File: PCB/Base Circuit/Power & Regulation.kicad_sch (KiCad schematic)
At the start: 25 parts, among them SW1_ESTOP SW_SPST

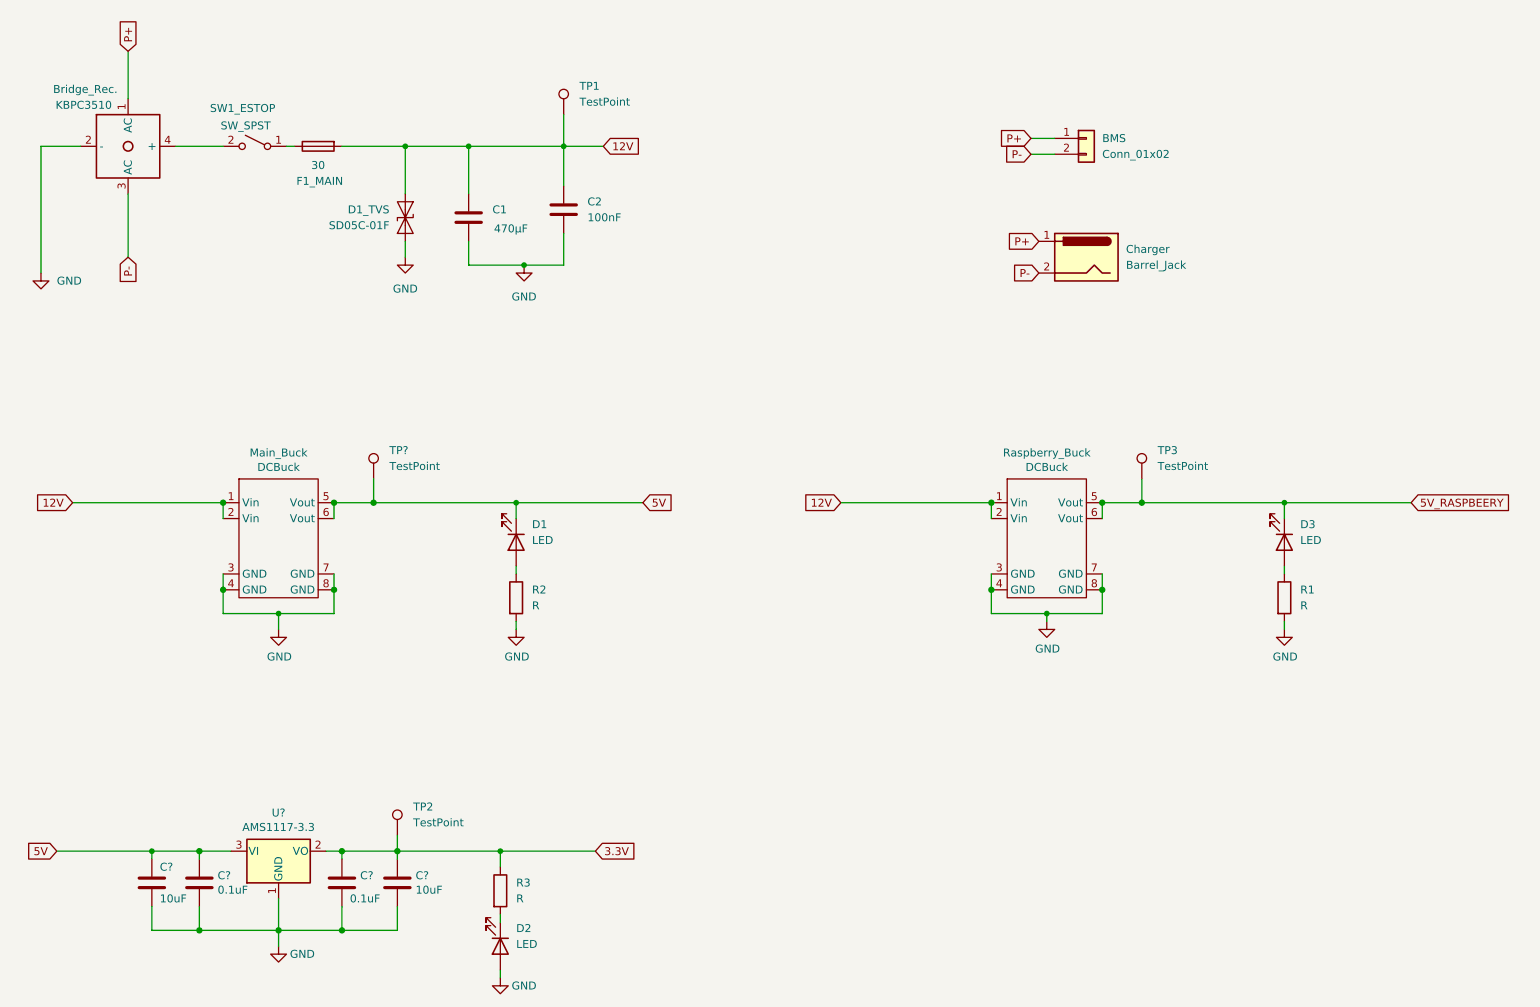
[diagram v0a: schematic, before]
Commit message: Final schematic updated
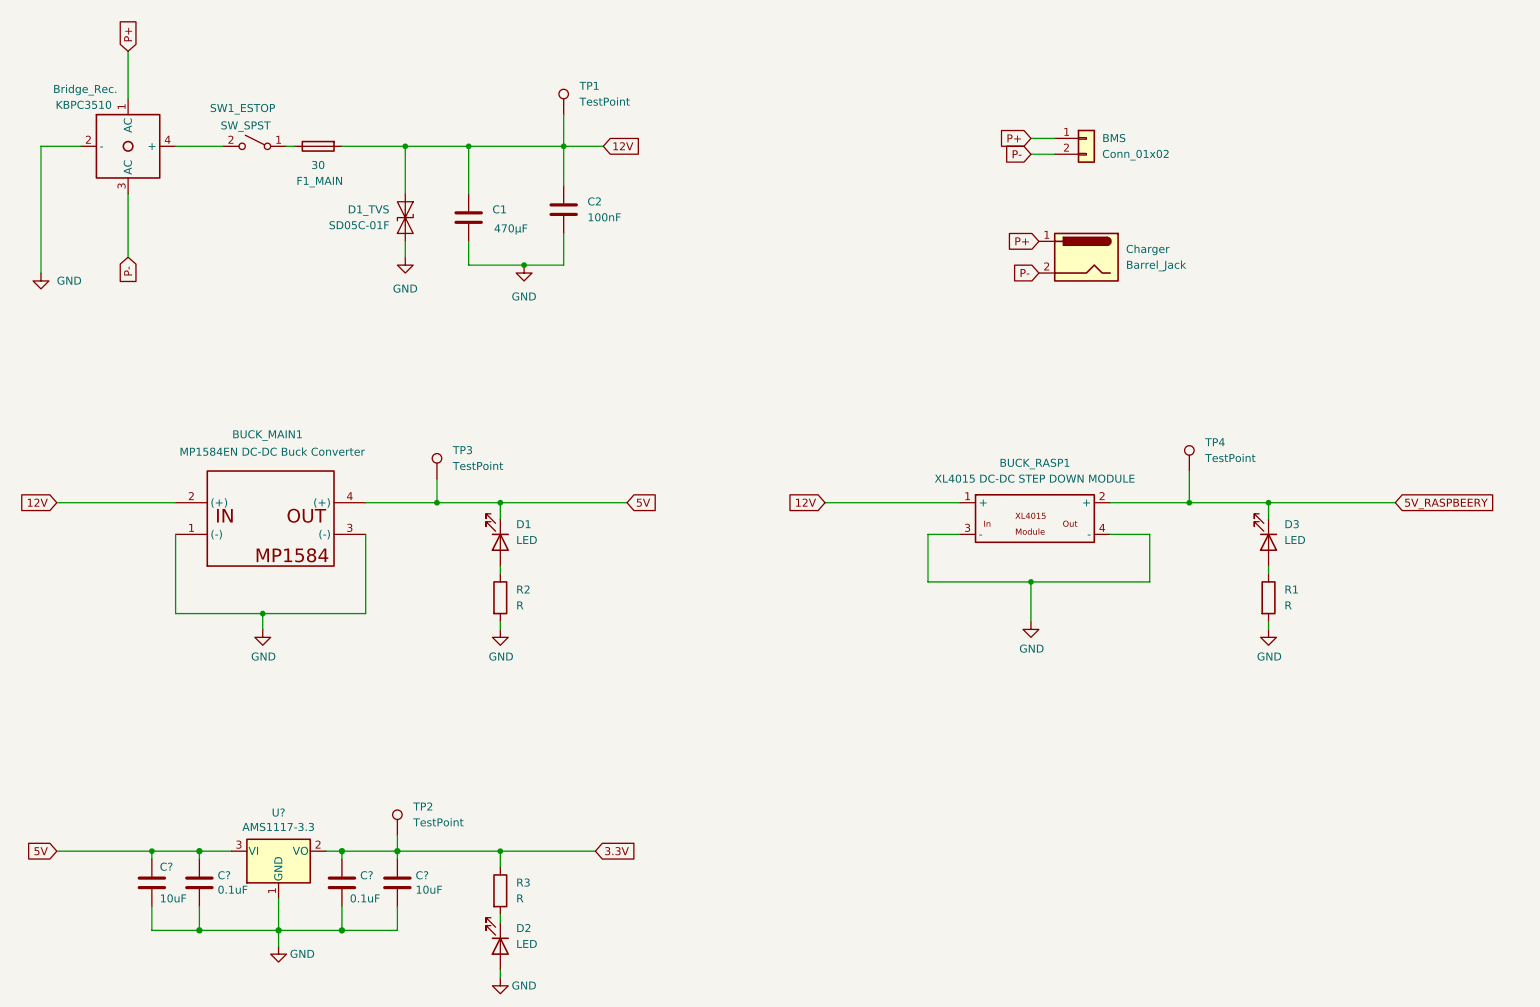
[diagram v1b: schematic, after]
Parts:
- removed Main_Buck, Raspberry_Buck: DCBuck, PrntrBoardV2:Buck2217, symbol BuckConverter:DCBuck
- removed TP?: TestPoint, symbol Connector:TestPoint
- added BUCK_MAIN1: MP1584EN DC-DC Buck Converter, Library:EBOOT MINI MP1584EN DC-DC BUCK CONVERTER ADJUSTABLE POWER STEP DOWN MODULE 24V TO 12V 9V 5V 3V, 6 PACK, symbol New_Library:eBoot Mini MP1584EN DC-DC Buck Converter Adjustable Power Step Down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
- added BUCK_RASP1: XL4015 DC-DC STEP DOWN MODULE, Library:XL4015 DC-DC STEP DOWN MODULE, symbol New_Library:XL4015 DC-DC STEP DOWN MODULE
- added TP3: TestPoint, TestPoint:TestPoint_THTPad_1.0x1.0mm_Drill0.5mm, symbol Connector:TestPoint
- D1, D3: footprint (none) -> LED_THT:LED_D3.0mm
- R1, R2: footprint (none) -> Resistor_THT:R_Axial_DIN0207_L6.3mm_D2.5mm_P7.62mm_Horizontal
- TP4: renamed from TP3; footprint (none) -> TestPoint:TestPoint_THTPad_1.0x1.0mm_Drill0.5mm
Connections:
- net 12V: now also BUCK_MAIN1.2 ((+)), BUCK_RASP1.1 (+)
- net 5V: now also BUCK_MAIN1.4 ((+)), TP3.1
- net 5V_RASPBEERY: now also BUCK_RASP1.2 (+)
- net GND: now also BUCK_MAIN1.1 ((-)), BUCK_MAIN1.3 ((-)), BUCK_RASP1.3 (-), BUCK_RASP1.4 (-)
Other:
- moved on the sheet: D3, R2, TP4
